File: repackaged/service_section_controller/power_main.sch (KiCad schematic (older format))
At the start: 22 parts, among them U201 TPS560430YF

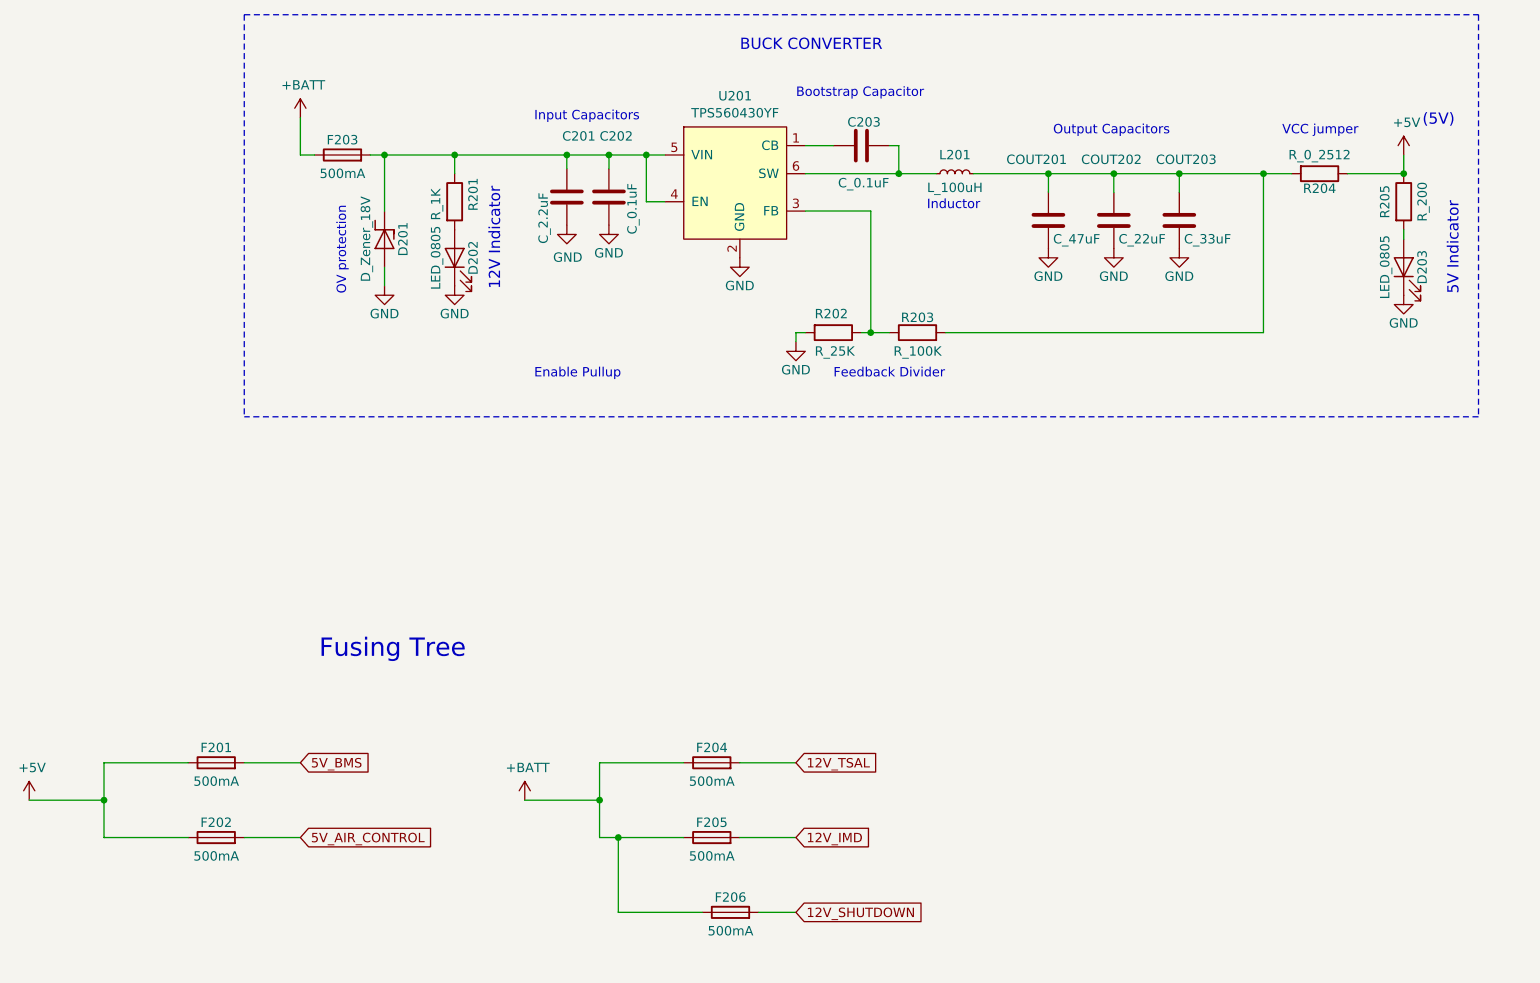
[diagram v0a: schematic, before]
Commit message: updated schematic
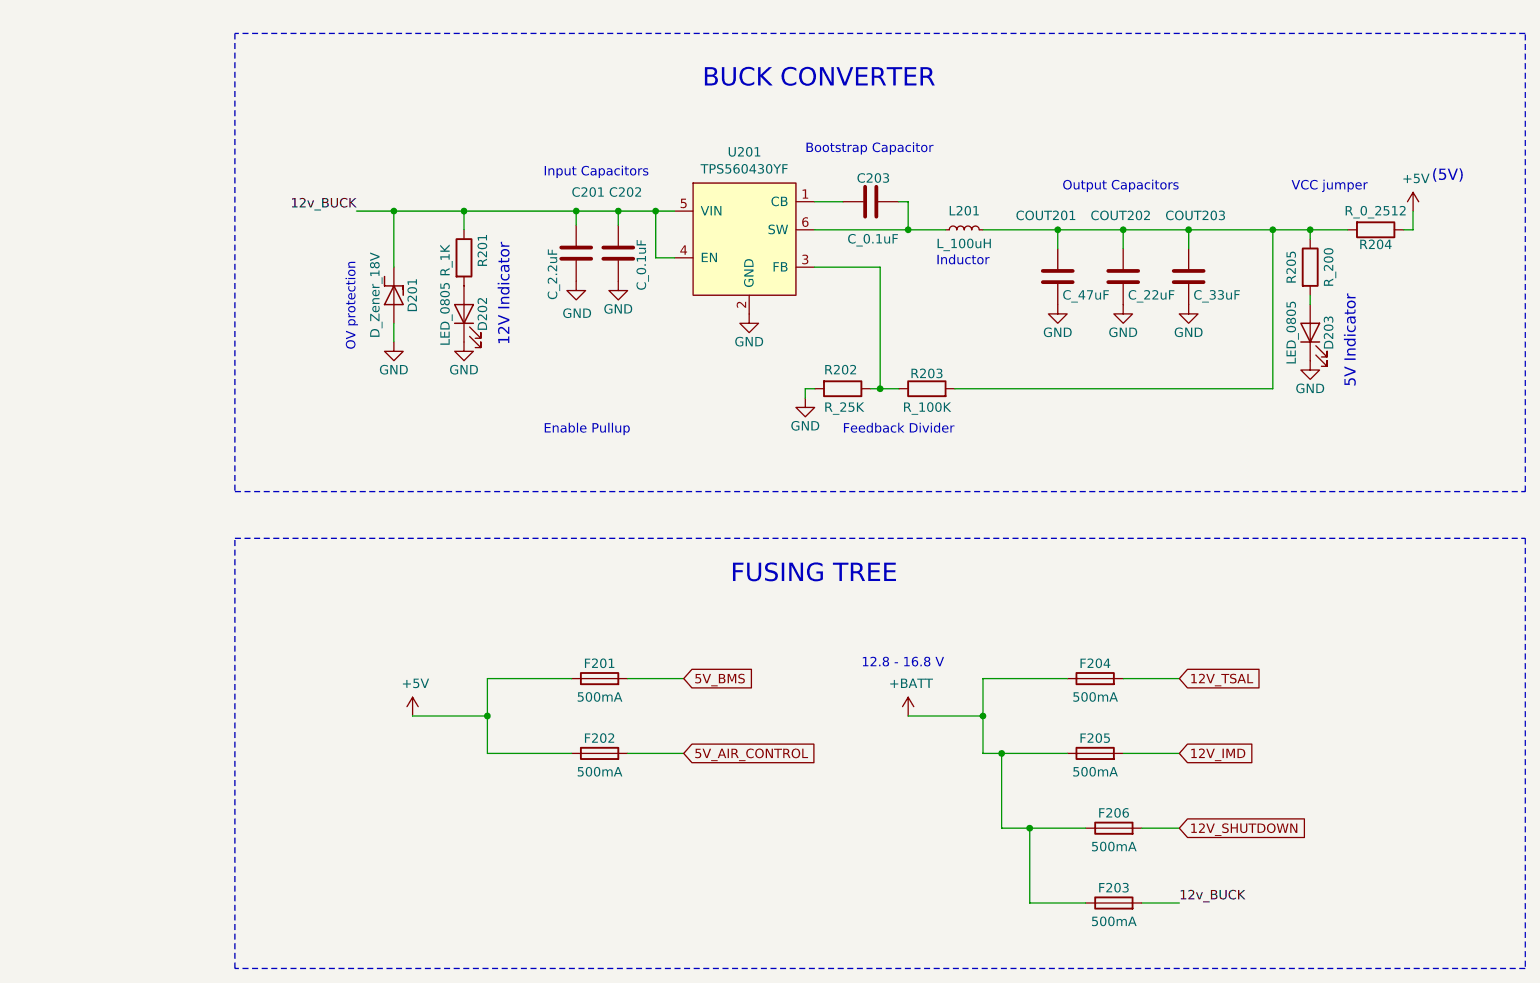
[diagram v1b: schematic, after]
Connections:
- net +5V: no longer R205.1
- net at COUT201.1, COUT202.1, COUT203.1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: now also R205.1
- net 12v_BUCK: now reaches C201.1, C202.1, D201.1 (K), F203.2, R201.1, U201.4 (EN), U201.5 (VIN)
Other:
- note added: "12.8 - 16.8 V"
- note added: "FUSING TREE"
- note removed: "Fusing Tree"
- moved on the sheet: C201, C202, C203, COUT201, COUT202, COUT203, D201, D202, D203, F201, F202, F203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
